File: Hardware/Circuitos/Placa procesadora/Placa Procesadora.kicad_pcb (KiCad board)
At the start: 2 copper layers, 46 x 45 mm, 26 parts, among them J1 Conn_01x02, J2 Conn_01x02, J7 Conn_01x02, U1 LM358

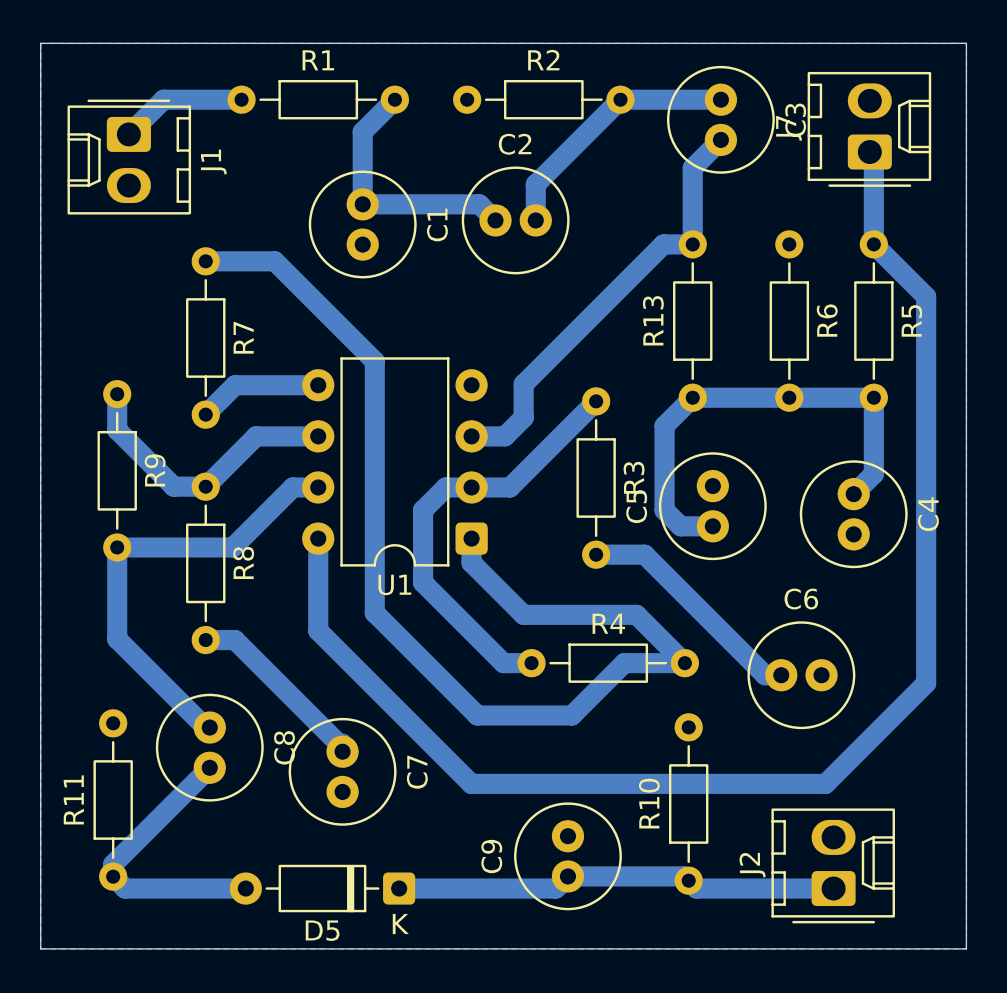
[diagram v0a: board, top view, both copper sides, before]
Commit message: Placa procesadora - Borde de placa
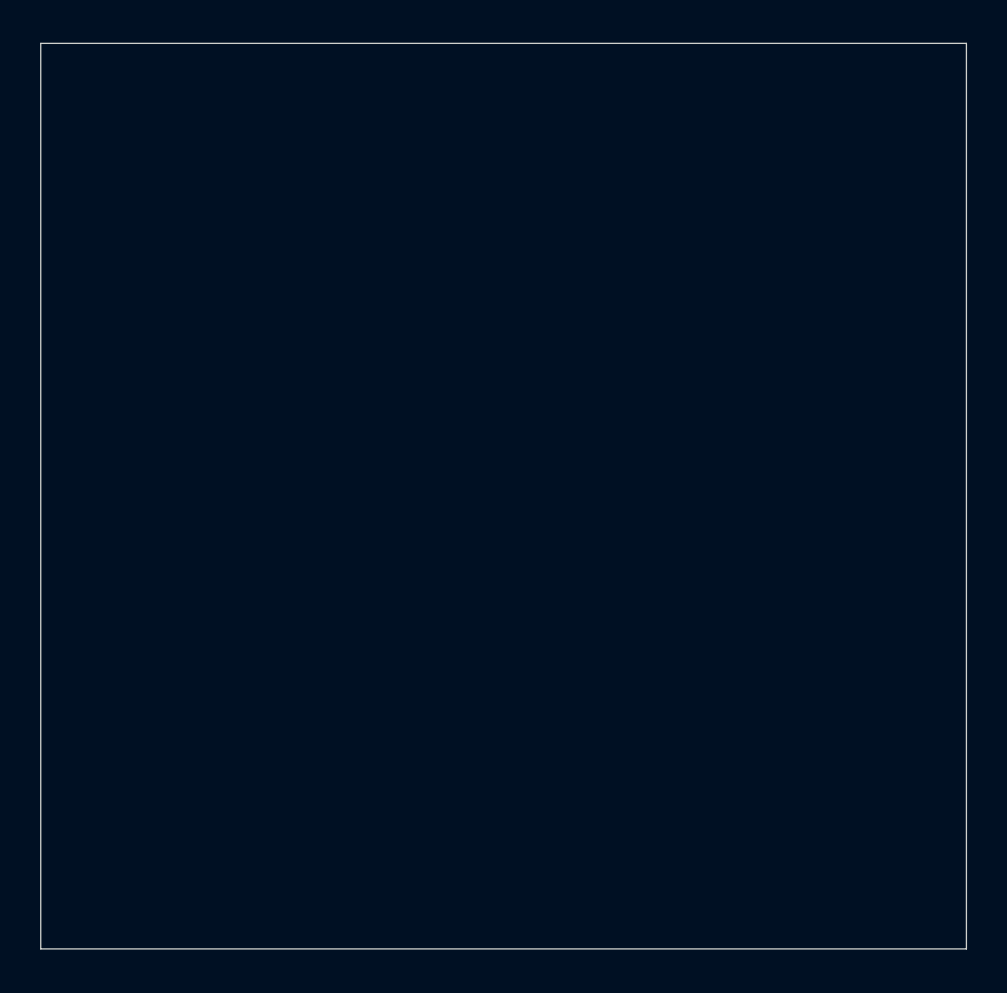
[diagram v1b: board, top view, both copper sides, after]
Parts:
- removed C1: 1nF, Capacitor_THT:C_Radial_D5.0mm_H11.0mm_P2.00mm
- removed C2: 390pF, Capacitor_THT:C_Radial_D5.0mm_H11.0mm_P2.00mm
- removed C3, C5, C8, C9: 100nF, Capacitor_THT:C_Radial_D5.0mm_H11.0mm_P2.00mm
- removed C4, C6, C7: 10uF, Capacitor_THT:C_Radial_D5.0mm_H11.0mm_P2.00mm
- removed D5: BAT-85, Diode_THT:D_DO-35_SOD27_P7.62mm_Horizontal
- removed J1, J2, J7: Conn_01x02, Connector_Molex:Molex_KK-254_AE-6410-02A_1x02_P2.54mm_Vertical
- removed R1: 3.9K, Resistor_THT:R_Axial_DIN0204_L3.6mm_D1.6mm_P7.62mm_Horizontal
- removed R10: 1M, Resistor_THT:R_Axial_DIN0204_L3.6mm_D1.6mm_P7.62mm_Horizontal
- removed R11: 100k, Resistor_THT:R_Axial_DIN0204_L3.6mm_D1.6mm_P7.62mm_Horizontal
- removed R13: 100K, Resistor_THT:R_Axial_DIN0204_L3.6mm_D1.6mm_P7.62mm_Horizontal
- removed R2, R5, R6: 10K, Resistor_THT:R_Axial_DIN0204_L3.6mm_D1.6mm_P7.62mm_Horizontal
- removed R3, R7, R8: 1K, Resistor_THT:R_Axial_DIN0204_L3.6mm_D1.6mm_P7.62mm_Horizontal
- removed R4, R9: 2.2K, Resistor_THT:R_Axial_DIN0204_L3.6mm_D1.6mm_P7.62mm_Horizontal
- removed U1: LM358, Package_DIP:DIP-8_W7.62mm
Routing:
- net /5V: track 67.6 -> 0.00 mm
- net Net-(R4-Pad2): track 55.4 -> 0.00 mm
- net Net-(C4-Pad1): track 23.1 -> 0.00 mm
- net Net-(C8-Pad1): track 22.2 -> 0.00 mm
- net Net-(D5-K): track 22.1 -> 0.00 mm
- net Net-(U1A-+): track 21.7 -> 0.00 mm
- net Net-(U1A--): track 21.5 -> 0.00 mm
- net Net-(D5-A): track 14.2 -> 0.00 mm
- net Net-(U1B--): track 14.0 -> 0.00 mm
- net Net-(C1-Pad1): track 12.8 -> 0.00 mm
- net Net-(C2-Pad2): track 12.7 -> 0.00 mm
- net Net-(C6-Pad1): track 11.7 -> 0.00 mm
- net Net-(C7-Pad1): track 8.93 -> 0.00 mm
- net Net-(J1-Pin_1): track 6.31 -> 0.00 mm
- net Net-(U1B-+): track 6.20 -> 0.00 mm
- removed copper zone on B.Cu, net Earth
